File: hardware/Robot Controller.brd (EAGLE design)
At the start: 51.7 x 41.3 mm, 17 parts, among them U1 ATMEGA328P_PDIP

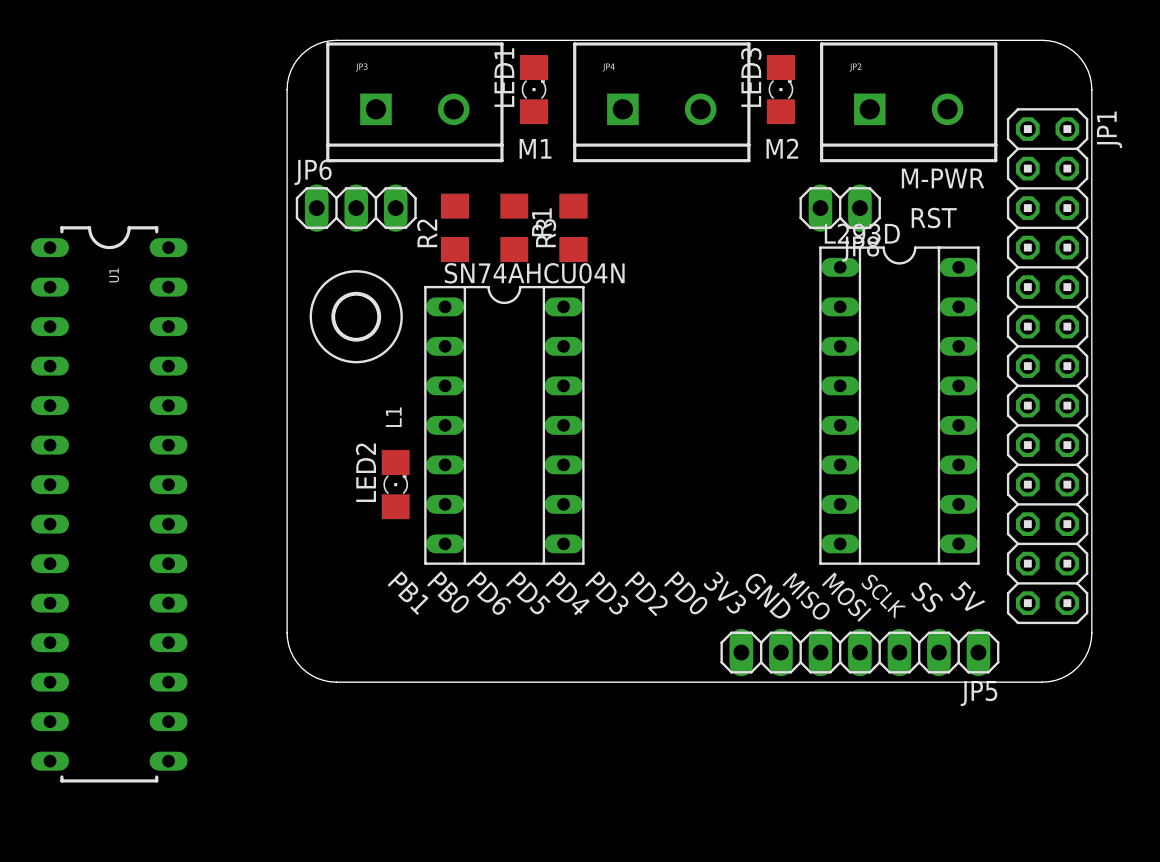
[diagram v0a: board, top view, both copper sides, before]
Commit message: rough routing
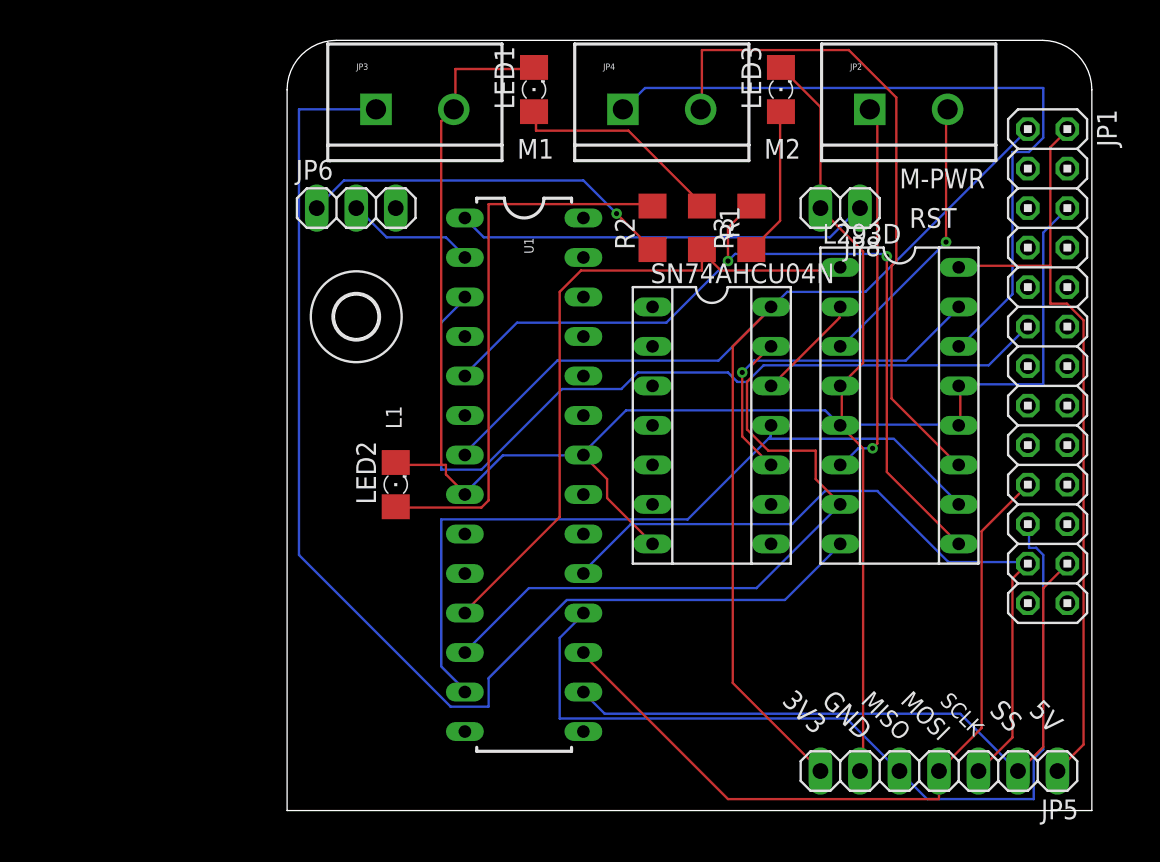
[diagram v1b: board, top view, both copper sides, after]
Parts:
- moved U1 26.7 mm to (57.1, 33.7)
- moved SN74AHCU04N 13.3 mm to (69.2, 36.8)
- moved R2 12.7 mm to (65.4, 49.5)
- moved R1 12.1 mm to (68.6, 49.5)
- moved R3 11.4 mm to (71.8, 49.5)
- moved JP5 9.16 mm to (83.8, 14.6)
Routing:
- net GND: track 0.00 -> 147.9 mm
- net 3.3V: track 0.00 -> 78.2 mm
- net N$10: track 0.00 -> 77.9 mm
- net MISO': track 0.00 -> 58.7 mm
- net M2PW': track 0.00 -> 55.1 mm, vias 0 -> 2
- net HOST': track 0.00 -> 53.8 mm
- net 5V: track 0.00 -> 49.9 mm
- net M2DR': track 0.00 -> 49.8 mm
- net MOSI': track 0.00 -> 49.4 mm
- net SCL': track 0.00 -> 47.5 mm
- net N$18: track 0.00 -> 47.1 mm
- net SS': track 0.00 -> 44.7 mm
- net M1PW': track 0.00 -> 43.9 mm
- net N$19: track 0.00 -> 43.2 mm
- net M1DR': track 0.00 -> 43.2 mm
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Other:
- board size 51.7 x 41.3 mm -> 51.7 x 49.5 mm
- board text added: "robot core rev 0.2"
- board text removed: "PB0"
- board text removed: "PB1"
- board text removed: "PD0"
- board text removed: "PD2"
- board text removed: "PD3"
- board text removed: "PD4"
- board text removed: "PD5"
- board text removed: "PD6"
- board text removed: "robot core rev 0.1"
